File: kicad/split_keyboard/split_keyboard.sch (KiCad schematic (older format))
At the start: 74 parts, among them J1 Conn_02x08_Odd_Even, SW1 SW_PUSH, SW10 SW_PUSH, SW11 SW_PUSH, SW12 SW_PUSH, SW13 SW_PUSH, SW14 SW_PUSH, SW15 SW_PUSH, SW16 SW_PUSH, SW17 SW_PUSH, SW18 SW_PUSH, SW19 SW_PUSH, SW2 SW_PUSH, SW20 SW_PUSH, SW21 SW_PUSH, SW22 SW_PUSH, SW23 SW_PUSH, SW24 SW_PUSH, SW25 SW_PUSH, SW26 SW_PUSH, SW27 SW_PUSH, SW28 SW_PUSH, SW29 SW_PUSH, SW3 SW_PUSH, SW30 SW_PUSH, SW31 SW_PUSH, SW32 SW_PUSH, SW33 SW_PUSH, SW34 SW_PUSH, SW35 SW_PUSH, SW36 SW_PUSH, SW4 SW_PUSH, SW5 SW_PUSH, SW6 SW_PUSH, SW7 SW_PUSH, SW8 SW_PUSH, SW9 SW_PUSH, U1 ESP32-DEVKITC-32D

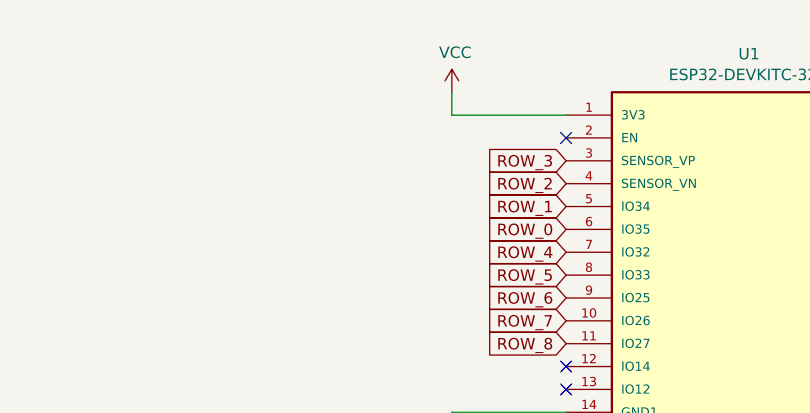
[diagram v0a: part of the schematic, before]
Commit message: complete lefthand pcb.
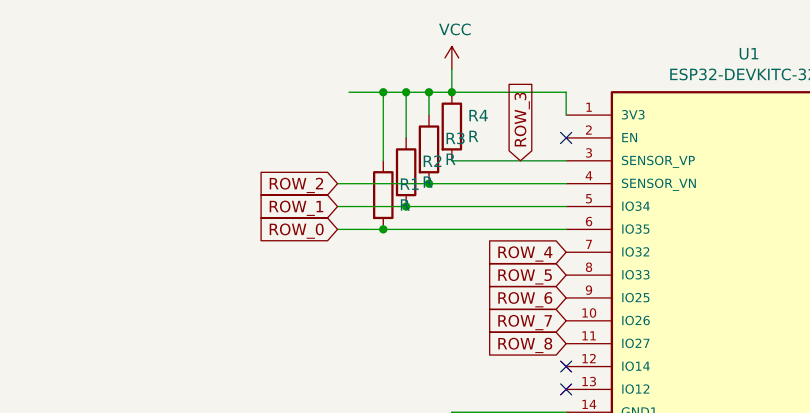
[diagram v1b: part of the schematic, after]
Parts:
- added R1, R2, R3, R4: R, Resistor_THT:R_Axial_DIN0207_L6.3mm_D2.5mm_P7.62mm_Horizontal, symbol Device:R
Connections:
- wire segments 96 -> 111
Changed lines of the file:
@@
 NoConn ~ 10100 1100
 NoConn ~ 10100 1200
-Text GLabel 8500 1200 0    50   Input ~ 0
+Text GLabel 7500 1200 0    50   Input ~ 0
 ROW_1
-Text GLabel 8500 1300 0    50   Input ~ 0
+Text GLabel 7500 1300 0    50   Input ~ 0
 ROW_0
-Text GLabel 8500 1000 0    50   Input ~ 0
+Text GLabel 8300 1000 1    50   Input ~ 0
 ROW_3
-Text GLabel 8500 1100 0    50   Input ~ 0
+Text GLabel 7500 1100 0    50   Input ~ 0
 ROW_2
 NoConn ~ 8500 2600
@@
 Wire Wire Line
 	8000 2100 8000 2700
-Wire Wire Line
-	8500 800  8000 800
-Wire Wire Line
-	8000 800  8000 700
 $Comp
 L power:VCC #PWR03
 U 1 1 5FAF706B
-P 8000 700
-F 0 "#PWR03" H 8000 550 50  0001 C CNN
-F 1 "VCC" H 8015 873 50  0000 C CNN
-F 2 "" H 8000 700 50  0001 C CNN
-F 3 "" H 8000 700 50  0001 C CNN
-	1    8000 700
+P 8000 600
+F 0 "#PWR03" H 8000 450 50  0001 C CNN
+F 1 "VCC" H 8015 773 50  0000 C CNN
+F 2 "" H 8000 600 50  0001 C CNN
+F 3 "" H 8000 600 50  0001 C CNN
+	1    8000 600
 	1    0    0    -1
 $EndComp
@@
 Text GLabel 3700 1400 0    50   Input ~ 0
 COL_1
+Wire Wire Line
+	7500 1100 7900 1100
+Wire Wire Line
+	8500 1200 7800 1200
+Wire Wire Line
+	7500 1300 7700 1300
+$Comp
+L Device:R R3
+U 1 1 5FB0ECDA
+P 7900 950
+F 0 "R3" H 7970 996 50  0000 L CNN
+F 1 "R" H 7970 905 50  0000 L CNN
+F 2 "Resistor_THT:R_Axial_DIN0207_L6.3mm_D2.5mm_P7.62mm_Horizontal" V 7830 950 50  0001 C CNN
+F 3 "~" H 7900 950 50  0001 C CNN
+	1    7900 950
+	1    0    0    -1
+$EndComp
+Connection ~ 7900 1100
+Wire Wire Line
+	7900 1100 8500 1100
+$Comp
+L Device:R R2
+U 1 1 5FB11470
+P 7800 1050
+F 0 "R2" H 7870 1096 50  0000 L CNN
+F 1 "R" H 7870 1005 50  0000 L CNN
+F 2 "Resistor_THT:R_Axial_DIN0207_L6.3mm_D2.5mm_P7.62mm_Horizontal" V 7730 1050 50  0001 C CNN
+F 3 "~" H 7800 1050 50  0001 C CNN
+	1    7800 1050
+	1    0    0    -1
+$EndComp
+Connection ~ 7800 1200
+Wire Wire Line
+	7800 1200 7500 1200
+$Comp
+L Device:R R1
+U 1 1 5FB12260
+P 7700 1150
+F 0 "R1" H 7770 1196 50  0000 L CNN
+F 1 "R" H 7770 1105 50  0000 L CNN
+F 2 "Resistor_THT:R_Axial_DIN0207_L6.3mm_D2.5mm_P7.62mm_Horizontal" V 7630 1150 50  0001 C CNN
+F 3 "~" H 7700 1150 50  0001 C CNN
+	1    7700 1150
+	1    0    0    -1
+$EndComp
+Connection ~ 7700 1300
+Wire Wire Line
+	7700 1300 8500 1300
+$Comp
+L Device:R R4
+U 1 1 5FB15C79
+P 8000 850
+F 0 "R4" H 8070 896 50  0000 L CNN
+F 1 "R" H 8070 805 50  0000 L CNN
+F 2 "Resistor_THT:R_Axial_DIN0207_L6.3mm_D2.5mm_P7.62mm_Horizontal" V 7930 850 50  0001 C CNN
+F 3 "~" H 8000 850 50  0001 C CNN
+	1    8000 850
+	1    0    0    -1
+$EndComp
+Wire Wire Line
+	8500 1000 8000 1000
+Wire Wire Line
+	8500 800  8500 700
+Wire Wire Line
+	8500 700  8000 700
+Connection ~ 8000 700
+Wire Wire Line
+	8000 700  7900 700
+Wire Wire Line
+	8000 700  8000 600
+Wire Wire Line
+	7900 800  7900 700
+Connection ~ 7900 700
+Wire Wire Line
+	7900 700  7800 700
+Wire Wire Line
+	7800 900  7800 700
+Connection ~ 7800 700
+Wire Wire Line
+	7800 700  7700 700
+Wire Wire Line
+	7700 1000 7700 700
+Connection ~ 7700 700
+Wire Wire Line
+	7700 700  7550 700
 $EndSCHEMATC

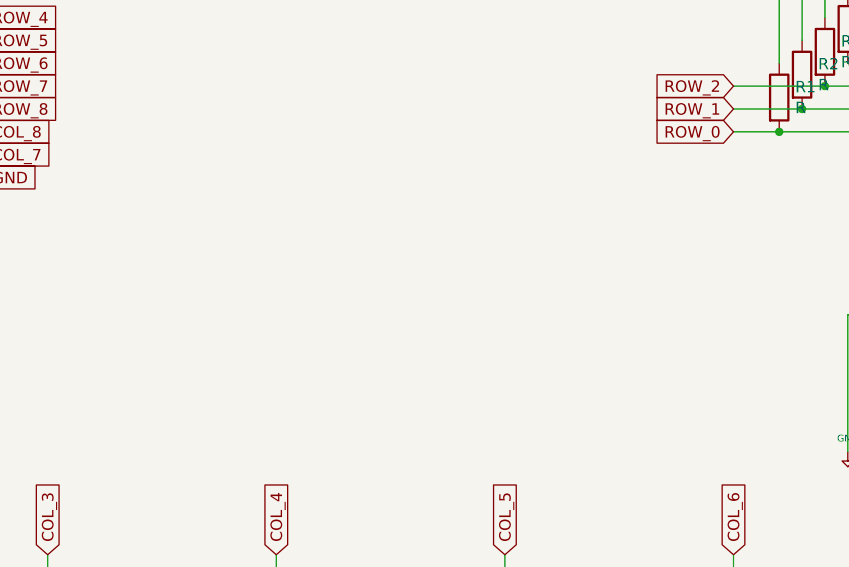
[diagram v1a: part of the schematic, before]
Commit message: complete to design pcb, and export gerber data.
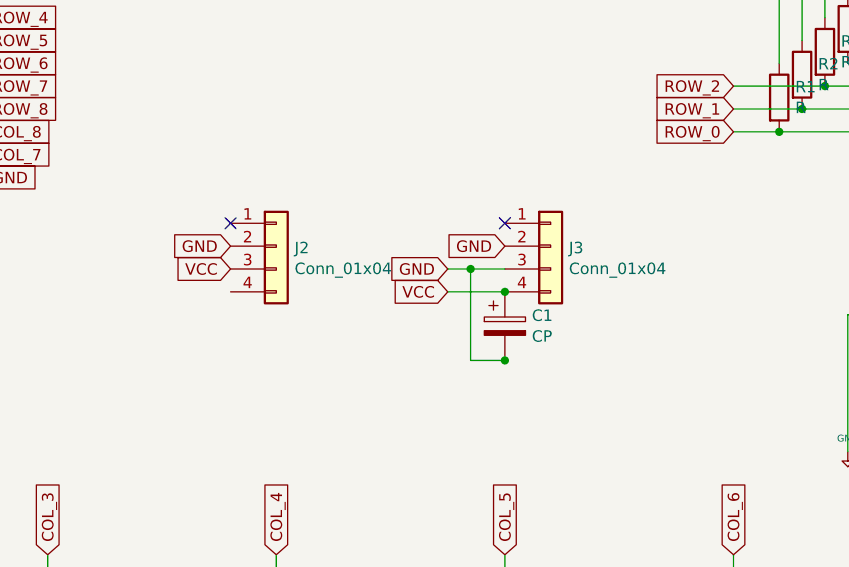
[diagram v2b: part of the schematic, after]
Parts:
- added C1: CP, Capacitor_THT:CP_Axial_L10.0mm_D4.5mm_P15.00mm_Horizontal, symbol Device:CP
- added J2, J3: Conn_01x04, Connector_PinSocket_2.54mm:PinSocket_1x04_P2.54mm_Vertical, symbol Connector_Generic:Conn_01x04
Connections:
- wire segments 111 -> 116
- no-connect marks 14 -> 16
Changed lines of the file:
@@
 Wire Wire Line
 	7700 700  7550 700
+$Comp
+L Connector_Generic:Conn_01x04 J2
+U 1 1 5FABFB3C
+P 5500 1800
+F 0 "J2" H 5580 1792 50  0000 L CNN
+F 1 "Conn_01x04" H 5580 1701 50  0000 L CNN
+F 2 "Connector_PinSocket_2.54mm:PinSocket_1x04_P2.54mm_Vertical" H 5500 1800 50  0001 C CNN
+F 3 "~" H 5500 1800 50  0001 C CNN
+	1    5500 1800
+	1    0    0    -1
+$EndComp
+$Comp
+L Connector_Generic:Conn_01x04 J3
+U 1 1 5FAC03DA
+P 6700 1800
+F 0 "J3" H 6780 1792 50  0000 L CNN
+F 1 "Conn_01x04" H 6780 1701 50  0000 L CNN
+F 2 "Connector_PinSocket_2.54mm:PinSocket_1x04_P2.54mm_Vertical" H 6700 1800 50  0001 C CNN
+F 3 "~" H 6700 1800 50  0001 C CNN
+	1    6700 1800
+	1    0    0    -1
+$EndComp
+Text GLabel 5300 1800 0    50   Input ~ 0
+GND
+Text GLabel 6500 1800 0    50   Input ~ 0
+GND
+Text GLabel 6250 1900 0    50   Input ~ 0
+GND
+Text GLabel 5300 1900 0    50   Input ~ 0
+VCC
+Text GLabel 6250 2000 0    50   Input ~ 0
+VCC
+NoConn ~ 5300 1700
+NoConn ~ 6500 1700
+Wire Wire Line
+	6250 1900 6350 1900
+Wire Wire Line
+	6500 2000 6250 2000
+Wire Wire Line
+	6350 2300 6350 1900
+Connection ~ 6350 1900
+Wire Wire Line
+	6350 1900 6500 1900
+Wire Wire Line
+	6500 2300 6350 2300
+Connection ~ 6500 2000
+$Comp
+L Device:CP C1
+U 1 1 5FB4051F
+P 6500 2150
+F 0 "C1" H 6618 2196 50  0000 L CNN
+F 1 "CP" H 6618 2105 50  0000 L CNN
+F 2 "Capacitor_THT:CP_Axial_L10.0mm_D4.5mm_P15.00mm_Horizontal" H 6538 2000 50  0001 C CNN
+F 3 "~" H 6500 2150 50  0001 C CNN
+	1    6500 2150
+	1    0    0    -1
+$EndComp
+Connection ~ 6500 2300
 $EndSCHEMATC
